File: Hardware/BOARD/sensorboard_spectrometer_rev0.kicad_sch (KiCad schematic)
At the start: 45 parts, among them IC1 CAT4101, IC2 CAT4101, U10 ADS1115IDGS, U11 TPS61088RHLT, U3 LILTGO touch, U4 W25Q16JVSS, U5 TLV9001IDCK, U6 MCP9808_MSOP, U7 TRANSLATOR-TXS0108E, U8 DS3231MZ, U9 LT3045xDD

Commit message: BOM
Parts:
- AS7331, U2: now left out of the parts list
- BAT_IN1, BAT_OU_LILYGO1, D1, D2, SWITCH_SPDT1: MP (none) -> 000561; Supplier (none) -> tinytronics
- BT1: MP (none) -> 001203; Supplier (none) -> tinytronics
- IC1, IC2: MP (none) -> CAT4104V-GT3; Supplier (none) -> farnell
- U3: MP (none) -> 004807
- U4: MP (none) -> W25Q16JVSSIQ; Supplier (none) -> digikey
- U7: MP (none) -> TXS0108EPWR; Supplier (none) -> digikey
- U9: MP (none) -> LT3045HDD#TRPBF; Supplier (none) -> digikey
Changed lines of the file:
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@@
 			)
 		)
-		(property "Supplier" ""
+		(property "Supplier" "tinytronics"
+			(at 181.61 189.23 0)
+			(effects
+				(font
+					(size 1.27 1.27)
+				)
+				(hide yes)
+			)
+		)
+		(property "MP" "000561"
 			(at 181.61 189.23 0)
 			(effects
@@
 			)
 		)
-		(property "Datasheet" "https://www.winbond.com/hq/support/documentation/levelOne.jsp?__locale=en&DocNo=DA00-W25Q16JV.1"
+		(property "Datasheet" "https://www.winbond.com/resource-files/w25q16jv%20spi%20revg%2003222018%20plus.pdf"
 			(at 372.11 129.54 0)
 			(effects
@@
 			)
 		)
-		(property "Supplier" ""
+		(property "Supplier" "digikey"
+			(at 372.11 129.54 0)
+			(effects
+				(font
+					(size 1.27 1.27)
+				)
+				(hide yes)
+			)
+		)
+		(property "MP" "W25Q16JVSSIQ"
 			(at 372.11 129.54 0)
 			(effects
@@
 			)
 		)
-		(property "Supplier" ""
+		(property "Supplier" "tinytronics"
+			(at 166.37 142.24 0)
+			(effects
+				(font
+					(size 1.27 1.27)
+				)
+				(hide yes)
+			)
+		)
+		(property "MP" "001203"
 			(at 166.37 142.24 0)
 			(effects
@@
 		(unit 1)
 		(exclude_from_sim no)
-		(in_bom yes)
+		(in_bom no)
 		(on_board yes)
 		(dnp no)
@@
 			)
 		)
-		(property "Supplier" ""
+		(property "Supplier" "tinytronics"
+			(at 237.49 175.26 0)
+			(effects
+				(font
+					(size 1.27 1.27)
+				)
+				(hide yes)
+			)
+		)
+		(property "MP" "000561"
 			(at 237.49 175.26 0)
 			(effects
@@
 		(unit 1)
 		(exclude_from_sim no)
-		(in_bom yes)
+		(in_bom no)
 		(on_board yes)
 		(dnp no)
@@
 			)
 		)
+		(property "MP" "004807"
+			(at 85.09 49.53 0)
+			(effects
+				(font
+					(size 1.27 1.27)
+				)
+				(hide yes)
+			)
+		)
 		(pin "8"
 		)
@@
 			)
 		)
-		(property "Supplier" ""
+		(property "Supplier" "farnell"
+			(at 313.69 223.52 0)
+			(effects
+				(font
+					(size 1.27 1.27)
+				)
+				(hide yes)
+			)
+		)
+		(property "MP" "CAT4104V-GT3"
 			(at 313.69 223.52 0)
 			(effects
@@
 			)
 		)
-		(property "Supplier" ""
+		(property "Supplier" "tinytronics"
+			(at 237.49 191.77 0)
+			(effects
+				(font
+					(size 1.27 1.27)
+				)
+				(hide yes)
+			)
+		)
+		(property "MP" "000561"
 			(at 237.49 191.77 0)
 			(effects
@@
 			)
 		)
-		(property "Supplier" ""
+		(property "Supplier" "farnell"
+			(at 311.15 177.8 0)
+			(effects
+				(font
+					(size 1.27 1.27)
+				)
+				(hide yes)
+			)
+		)
+		(property "MP" "CAT4104V-GT3"
 			(at 311.15 177.8 0)
 			(effects
@@
 			)
 		)
-		(property "Supplier" ""
+		(property "Supplier" "tinytronics"
+			(at 326.39 177.8 0)
+			(effects
+				(font
+					(size 1.27 1.27)
+				)
+				(hide yes)
+			)
+		)
+		(property "MP" "000561"
 			(at 326.39 177.8 0)
 			(effects
@@
 			)
 		)
-		(property "Datasheet" "https://www.analog.com/media/en/technical-documentation/data-sheets/3045fa.pdf"
+		(property "Datasheet" "https://www.analog.com/media/en/technical-documentation/data-sheets/LT3045.pdf"
 			(at 82.55 179.07 0)
 			(effects
@@
 			)
 		)
-		(property "Supplier" ""
+		(property "Supplier" "digikey"
+			(at 82.55 179.07 0)
+			(effects
+				(font
+					(size 1.27 1.27)
+				)
+				(hide yes)
+			)
+		)
+		(property "MP" "LT3045HDD#TRPBF"
 			(at 82.55 179.07 0)
 			(effects
@@
 			)
 		)
-		(property "Supplier" ""
+		(property "Supplier" "tinytronics"
+			(at 328.93 223.52 0)
+			(effects
+				(font
+					(size 1.27 1.27)
+				)
+				(hide yes)
+			)
+		)
+		(property "MP" "000561"
 			(at 328.93 223.52 0)
 			(effects
@@
 			)
 		)
-		(property "Datasheet" "https://www.ti.com/lit/ds/symlink/txs0108e.pdf"
+		(property "Datasheet" "https://www.ti.com/lit/ds/symlink/txs0108e.pdf?ts=1763832768609"
 			(at 300.99 125.73 0)
 			(effects
@@
 			)
 		)
-		(property "Supplier" ""
+		(property "Supplier" "digikey"
+			(at 300.99 125.73 0)
+			(effects
+				(font
+					(size 1.27 1.27)
+				)
+				(hide yes)
+			)
+		)
+		(property "MP" "TXS0108EPWR"
 			(at 300.99 125.73 0)
 			(effects

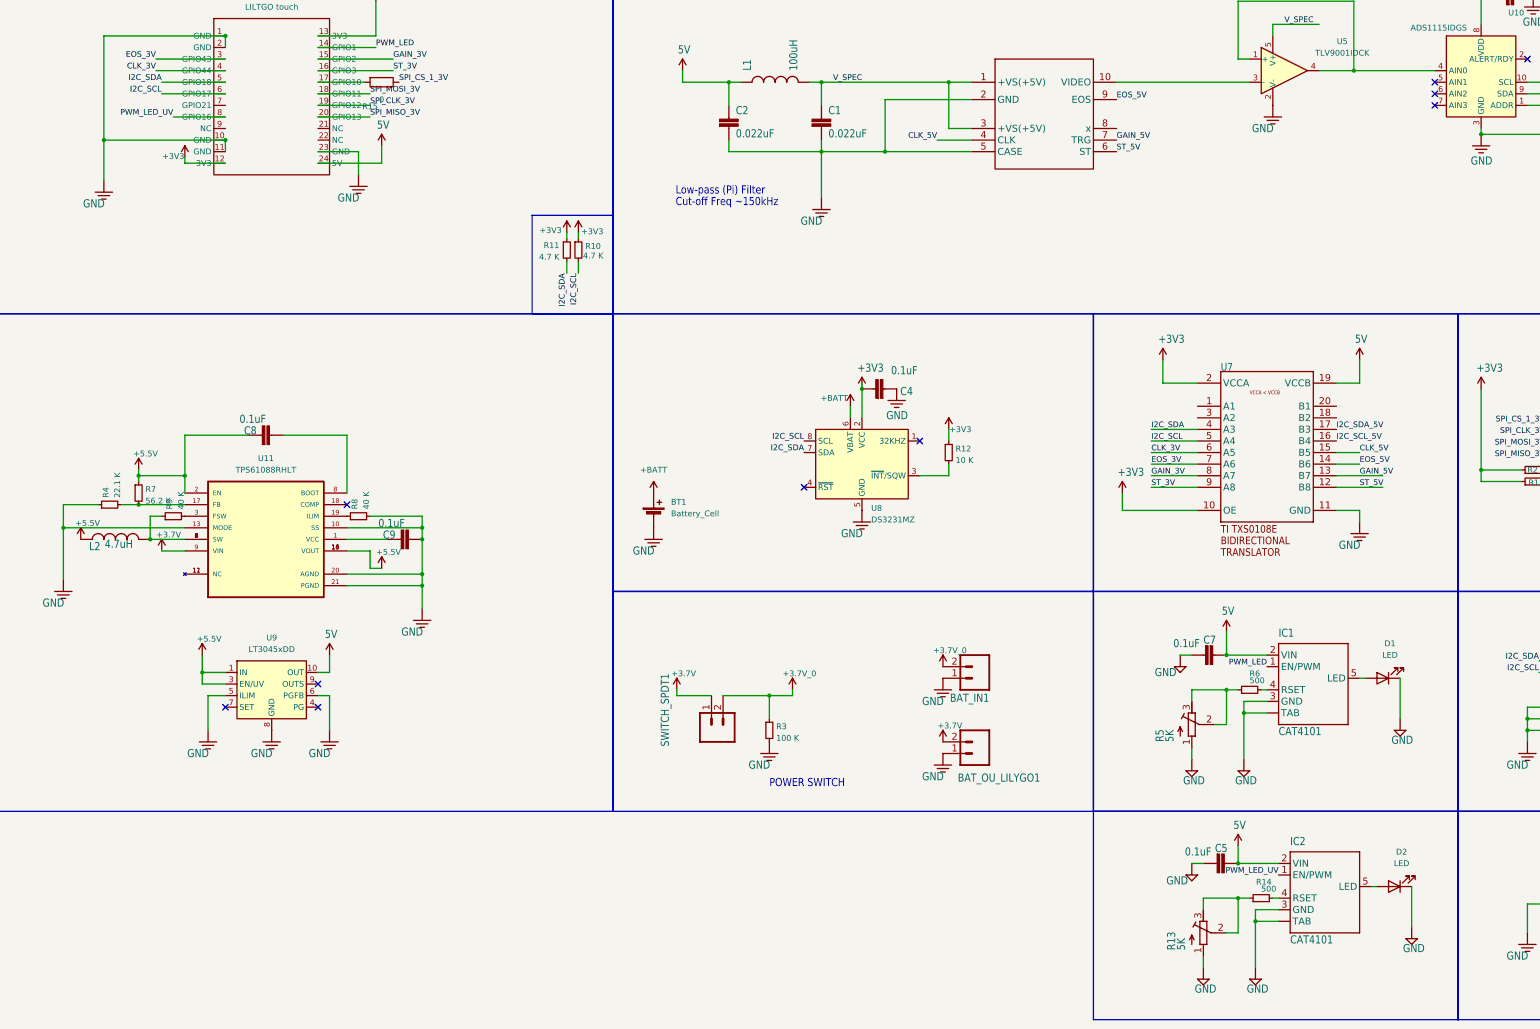
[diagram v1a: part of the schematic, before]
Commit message: before maked
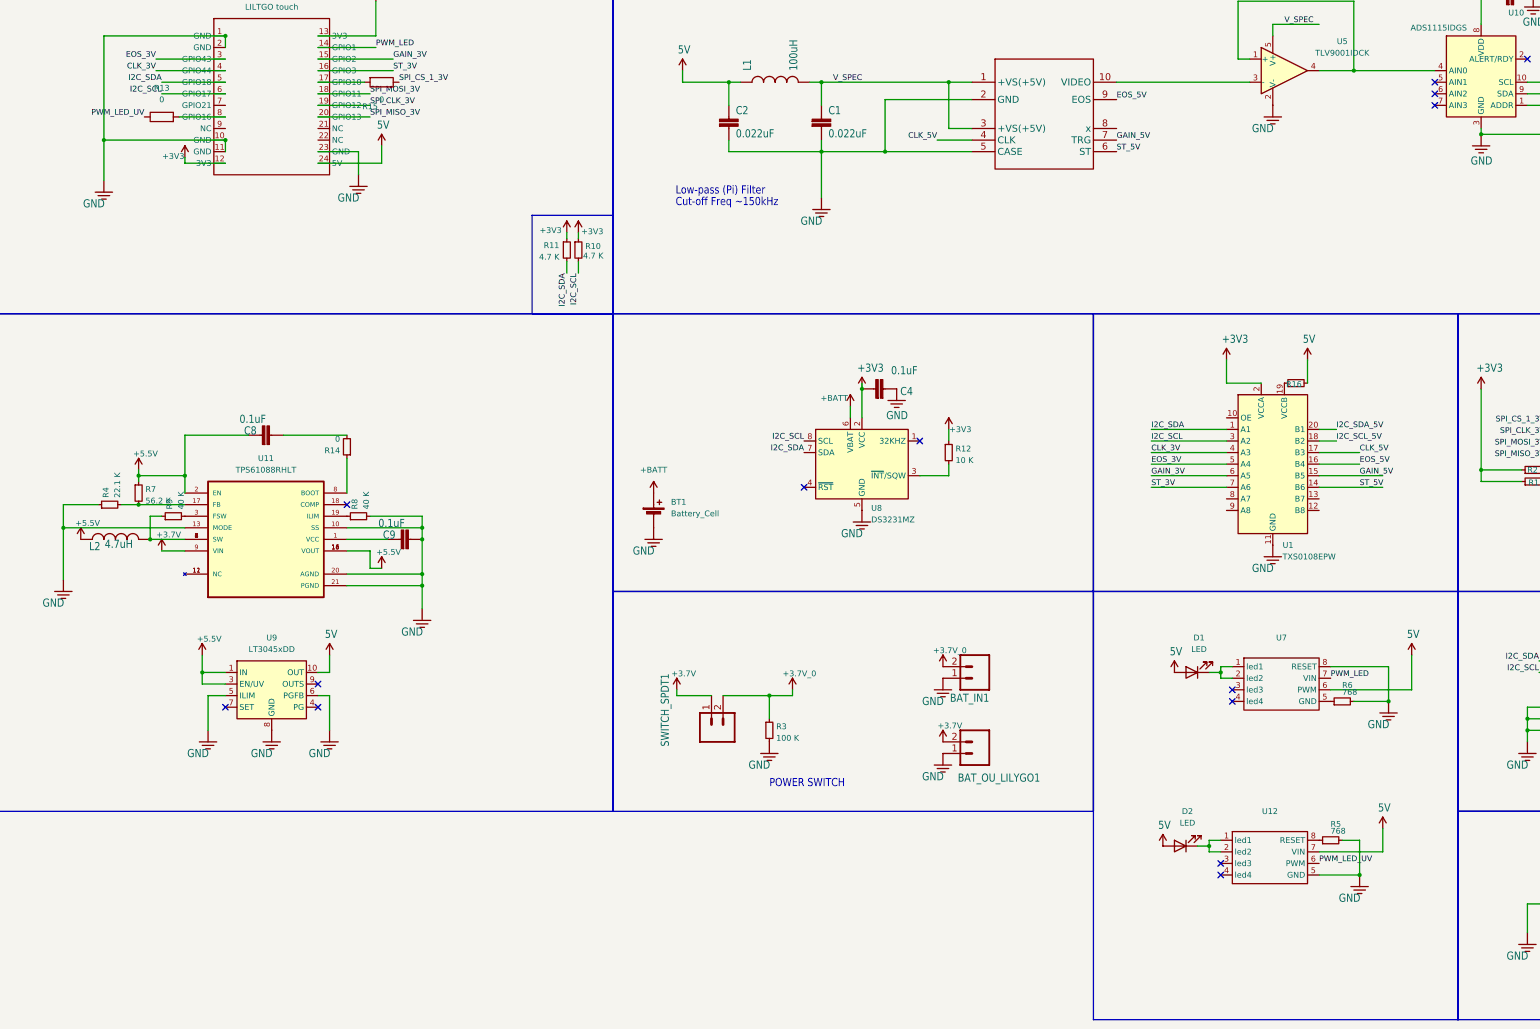
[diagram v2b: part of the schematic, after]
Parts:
- removed C5, C7: 0.1uF, Capacitor_SMD:C_0603_1608Metric, symbol sensorboard_spectrometer_rev0-eagle-import:notes_mark5_CAP0603
- removed IC1, IC2: CAT4101, Package_TO_SOT_SMD:TO-263-5_TabPin6, symbol F9ZYROSHVXBZZL3-eagle-import:CAT4101
- removed R13, R5: 5K, Potentiometer_THT:Potentiometer_Runtron_RM-065_Vertical, symbol F9ZYROSHVXBZZL3-eagle-import:R-TRIMM64W
- removed U7: TRANSLATOR-TXS0108E, Package_SO:TSSOP-20_4.4x5mm_P0.5mm, symbol sensorboard_spectrometer_rev0-eagle-import:TRANSLATOR-TXS0108E
- added R13: 0, Resistor_SMD:R_0603_1608Metric, symbol Device:R
- added R16: 0, Resistor_SMD:R_0603_1608Metric, symbol Device:R_Small
- added R5: 768, Resistor_SMD:R_0603_1608Metric, symbol Device:R_Small
- added U1: TXS0108EPW, Package_SO:TSSOP-20_4.4x6.5mm_P0.65mm, symbol Logic_LevelTranslator:TXS0108EPW
- added U12, U7: ~, Package_SO:PowerIntegrations_SO-8, symbol oTROSs:cat4104v
- C1, C2: MP C0603C223K5RACTU -> C0603C104K3RACTU; Supplier digikey -> farnell
- C10, C3, C4, C8, C9, L1, L2, R1, R12, R2, R3, U8, U9: Supplier digikey -> farnell
- R10, R11: MP M55342K12B4E75RS2 -> ERJ3EKF4751V; Supplier digikey -> farnell
- R14: value 500 -> 0; MP M55342K12B590DRS2 -> WR06X3922FTL; Supplier digikey -> farnell
- R15: MP M55342K12B4E75RS2 -> MCWR06X000 PTL; Supplier digikey -> farnell
- R4: MP M55342K12B20E0RS2 -> ERA3AEB203V; Supplier digikey -> farnell
- R6: value 500 -> 768; MP M55342K12B590DRS2 -> RC0603FR-07590RL; Supplier digikey -> mouser
- R7: MP M55342K12B56E2RWB -> ERA3ARB5622V; Supplier digikey -> mouser
- R8, R9: MP M55342K12B39E2RS2 -> WR06X3922FTL; Supplier digikey -> farnell
- U10: MP ADS1115IDGS -> ADS1115BQDGSRQ1; Supplier digikey -> farnell
- U11, U4, U5: Supplier digikey -> mouser
- U6: MP MCP9808_MSOP -> 579-MCP9808-E/MS; Supplier digikey -> mouser
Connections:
- net +3V3: now also U1.2 (VCCA)
- net 5V: now also D1.2 (A), D2.2 (A), R16.2, U12.7 (VIN), U7.6 (PWM)
- net CLK_3V: now also U1.4 (A3)
- net CLK_5V: now also U1.17 (B3)
- net EOS_3V: now also U1.5 (A4)
- net EOS_5V: now also U1.16 (B4)
- net GAIN_3V: now also U1.6 (A5)
- net GAIN_5V: now also U1.15 (B5)
- net GND: now also R6.2, R5.2, U1.11 (GND), U12.5 (GND), U7.8 (RESET); no longer D1.1 (K), D2.1 (K)
- net I2C_SCL: now also U1.3 (A2)
- net I2C_SCL_5V: now also U1.18 (B2)
- net I2C_SDA: now also U1.1 (A1)
- net I2C_SDA_5V: now also U1.20 (B1)
- net PWM_LED: now also U7.7 (VIN)
- net PWM_LED_UV: now also R13.1, U12.6 (PWM); no longer U3.8 (GPIO16)
- net ST_3V: now also U1.7 (A6)
- net ST_5V: now also U1.14 (B6)
- net at R14.1: now also U11.8 (BOOT)
- net at R14.2: now also C8.2
- net at R6.1: now also U7.5 (GND)
- new net: D2.1 (K), U12.1 (led1), U12.2 (led2)
- new net: R5.1, U12.8 (RESET)
- new net: D1.1 (K), U7.1 (led1), U7.2 (led2)
- new net: R13.2, U3.8 (GPIO16)
- new net: R16.1, U1.19 (VCCB)
- no-connect marks 15 -> 19
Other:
- moved on the sheet: D1, D2, R6

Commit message: alex suggest changes
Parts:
- C3: footprint Capacitor_SMD:C_0603_1608Metric -> Capacitor_SMD:C_1206_3216Metric
- R11, R13, R15, R16, R2: footprint Resistor_SMD:R_0603_1608Metric -> Resistor_SMD:R_1206_3216Metric
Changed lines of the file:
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@@
 			)
 		)
-		(property "Footprint" "Resistor_SMD:R_0603_1608Metric"
+		(property "Footprint" "Resistor_SMD:R_1206_3216Metric"
 			(at 359.41 132.08 0)
 			(effects
@@
 			)
 		)
-		(property "Footprint" "Capacitor_SMD:C_0603_1608Metric"
+		(property "Footprint" "Capacitor_SMD:C_1206_3216Metric"
 			(at 377.19 110.49 0)
 			(effects
@@
 			)
 		)
-		(property "Footprint" "Resistor_SMD:R_0603_1608Metric"
+		(property "Footprint" "Resistor_SMD:R_1206_3216Metric"
 			(at 147.32 83.82 0)
 			(effects
@@
 			)
 		)
-		(property "Footprint" "Resistor_SMD:R_0603_1608Metric"
+		(property "Footprint" "Resistor_SMD:R_1206_3216Metric"
 			(at 106.68 45.212 90)
 			(effects
@@
 			)
 		)
-		(property "Footprint" "Resistor_SMD:R_0603_1608Metric"
+		(property "Footprint" "Resistor_SMD:R_1206_3216Metric"
 			(at 58.42 56.388 90)
 			(effects
@@
 			)
 		)
-		(property "Footprint" "Resistor_SMD:R_0603_1608Metric"
+		(property "Footprint" "Resistor_SMD:R_1206_3216Metric"
 			(at 307.34 113.03 0)
 			(effects
